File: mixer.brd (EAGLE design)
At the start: 23 x 40 mm, 21 parts, among them U2 SA602AD8-SOIC

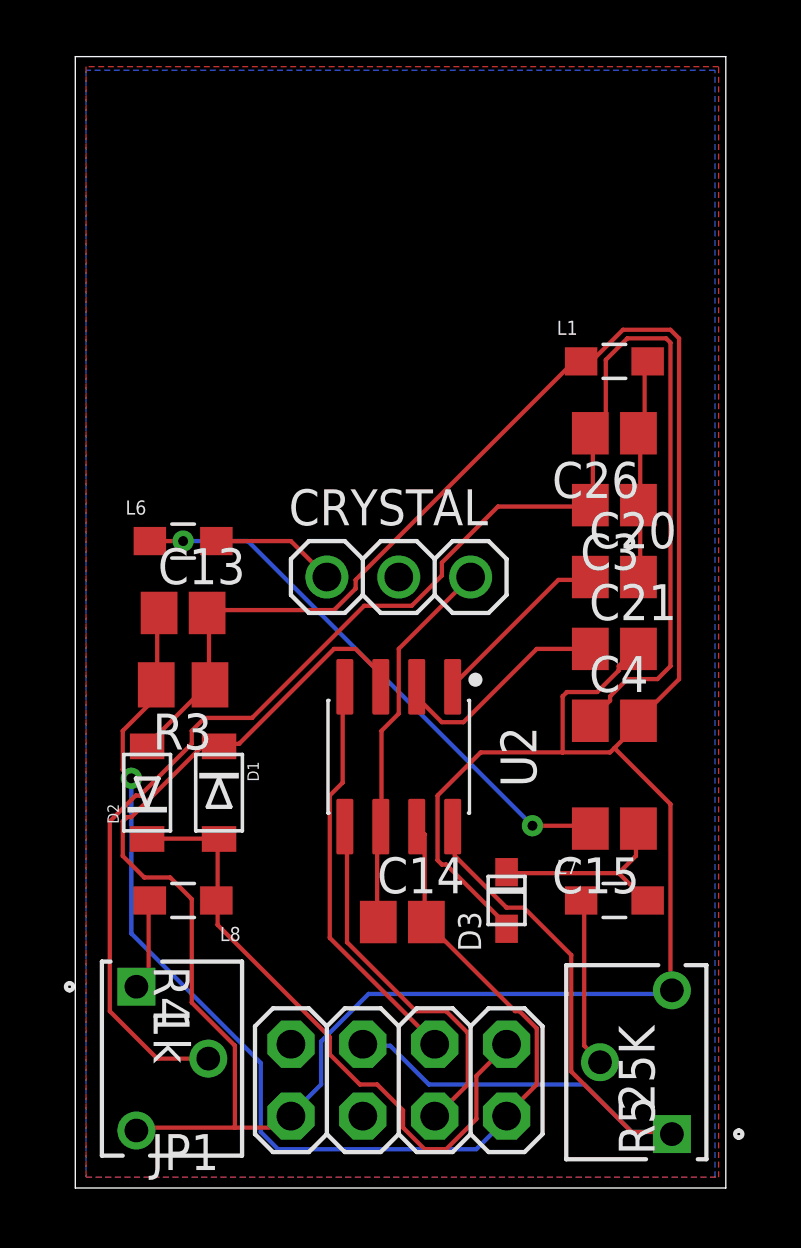
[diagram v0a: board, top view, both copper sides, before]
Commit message: updating layouts and parts
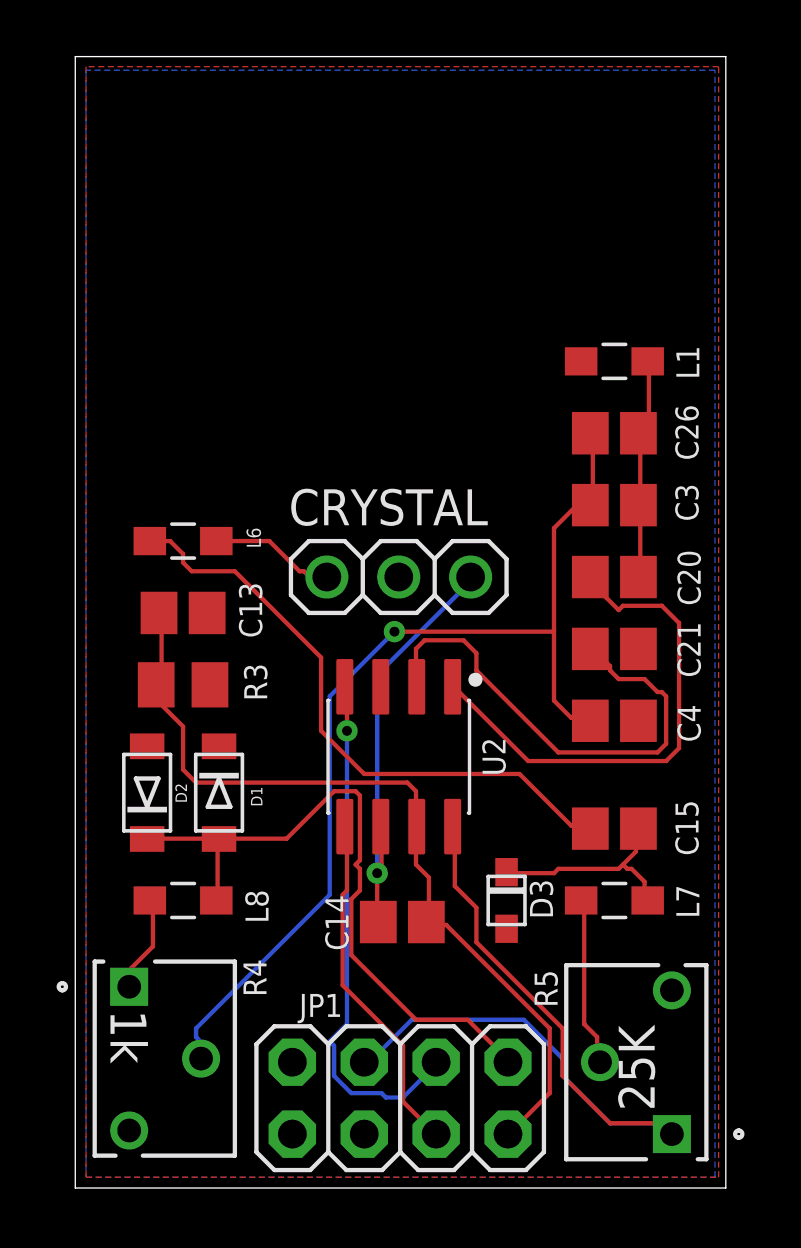
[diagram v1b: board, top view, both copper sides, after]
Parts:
- moved JP1 0.64 mm to (11.5, 3.17)
- moved R4 0.25 mm to (1.91, 7.11)
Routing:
- net GND: track 117.4 -> 0.00 mm
- net N$5: track 56.3 -> 35.7 mm, vias 0 -> 1
- net ANT_OUT: track 42.9 -> 29.7 mm, vias 1 -> 0
- net N$1: track 6.50 -> 17.9 mm
- net N$2: track 7.98 -> 17.6 mm
- net OUT_A: track 14.4 -> 18.6 mm, vias 0 -> 1
- net N$4: track 13.6 -> 15.3 mm, vias 0 -> 1
- net N$16: track 19.8 -> 21.5 mm, vias 2 -> 0
- net 6V_DC: track 27.5 -> 28.7 mm
- net ANT_IN: track 22.3 -> 23.5 mm
- net OUT_B: track 13.1 -> 12.3 mm
